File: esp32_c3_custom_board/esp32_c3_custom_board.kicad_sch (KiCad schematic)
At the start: 44 parts, among them IC1 ESP32-C3, IC2 GD25Q16CTEGR, J1 USB-C Connector, U1 ESD Protection, U2 SPX3819M5-L-3-3, Y1 830108208709_crystal

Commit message: .
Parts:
- IC1: footprint QFN50P500X500X90-33N-D -> ESP32-C3:QFN50P500X500X90-33N-D
- IC2: footprint SOIC127P600X175-8N -> GD25Q16CTEGR:SOIC127P600X175-8N
- J1: footprint GSB1C41110SSHR -> GSB1C41110SSHR:GSB1C41110SSHR
- S1: footprint 434781025816 -> 434781025816:434781025816
- U1: footprint Package_TO_SOT_SMD:SOT-666 -> USBLC6-2SC6:SOT95P280X145-6N
- U2: footprint Package_TO_SOT_SMD:SOT-23-5 -> SPX3819M5-L-3-3_TR:SOT95P280X145-5N
- Y1: footprint 830108208709 -> 830108208709:830108208709
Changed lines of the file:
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@@
       (effects (font (size 1.27 1.27)))
     )
-    (property "Footprint" "QFN50P500X500X90-33N-D" (at 240.03 154.61 0)
+    (property "Footprint" "ESP32-C3:QFN50P500X500X90-33N-D" (at 240.03 154.61 0)
       (effects (font (size 1.27 1.27)) (justify left top) hide)
     )
@@
       (effects (font (size 1 1)))
     )
-    (property "Footprint" "Package_TO_SOT_SMD:SOT-23-5" (at 115.57 28.575 0)
+    (property "Footprint" "SPX3819M5-L-3-3_TR:SOT95P280X145-5N" (at 115.57 28.575 0)
       (effects (font (size 1.27 1.27)) hide)
     )
@@
       (effects (font (size 1.27 1.27)) (justify left))
     )
-    (property "Footprint" "Package_TO_SOT_SMD:SOT-666" (at 97.79 172.72 0)
+    (property "Footprint" "USBLC6-2SC6:SOT95P280X145-6N" (at 97.79 172.72 0)
       (effects (font (size 1.27 1.27)) hide)
     )
@@
       (effects (font (size 1.27 1.27)))
     )
-    (property "Footprint" "830108208709" (at 246.38 233.35 0)
+    (property "Footprint" "830108208709:830108208709" (at 246.38 233.35 0)
       (effects (font (size 1.27 1.27)) (justify left top) hide)
     )
@@
       (effects (font (size 1.27 1.27)))
     )
-    (property "Footprint" "GSB1C41110SSHR" (at 68.58 223.19 0)
+    (property "Footprint" "GSB1C41110SSHR:GSB1C41110SSHR" (at 68.58 223.19 0)
       (effects (font (size 1.27 1.27)) (justify left top) hide)
     )
@@
       (effects (font (size 1.27 1.27)) (justify left))
     )
-    (property "Footprint" "434781025816" (at 196.85 187.63 0)
+    (property "Footprint" "434781025816:434781025816" (at 196.85 187.63 0)
       (effects (font (size 1.27 1.27)) (justify left top) hide)
     )
@@
       (effects (font (size 1.27 1.27)))
     )
-    (property "Footprint" "SOIC127P600X175-8N" (at 68.58 185.09 0)
-      (effects (font (size 1.27 1.27)) (justify left top) hide)
-    )
+    (property "Footprint" "GD25Q16CTEGR:SOIC127P600X175-8N" (at 68.58 185.09 0)
+      (effects (font (size 1.27 1.27)) (justify left top) hide)
+    )

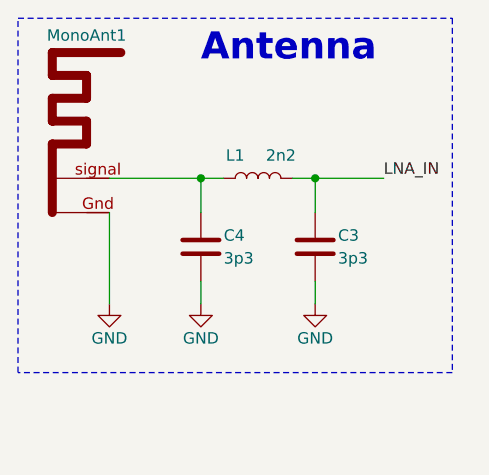
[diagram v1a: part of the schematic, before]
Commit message: .
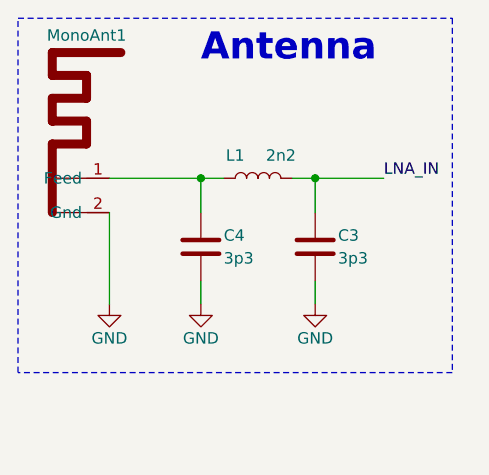
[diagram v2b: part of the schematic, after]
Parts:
- C1, C10, C11, C12, C13, C14, C15, C16, C2, C3, C4, C5, C6, C7, C8, C9: footprint (none) -> Capacitor_SMD:C_0201_0603Metric
- D1, D2: footprint (none) -> ASCKCF00-AP5R5010402:ASCKCF00AP5R5010402
- L1, L2: footprint (none) -> Inductor_SMD:L_0603_1608Metric
- MonoAnt1: footprint (none) -> Footprint_Lib:Mono_Ant
- R1, R10, R11, R12, R13, R14, R15, R2, R3, R4, R5, R6, R7, R8, R9: footprint (none) -> Resistor_SMD:R_0201_0603Metric
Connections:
- net GND: now also MonoAnt1.2 (Gnd); no longer MonoAnt1.Gnd
- net at C4.1, L1.1: now also MonoAnt1.1 (Feed); no longer MonoAnt1.signal
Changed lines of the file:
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@@
       (effects (font (size 1.27 1.27)) (justify left))
     )
-    (property "Footprint" "" (at 154.432 87.63 90)
+    (property "Footprint" "Resistor_SMD:R_0201_0603Metric" (at 154.432 87.63 90)
       (effects (font (size 1.27 1.27)) hide)
     )
@@
       (effects (font (size 1.27 1.27)) (justify left))
     )
-    (property "Footprint" "" (at 75.8952 45.72 0)
+    (property "Footprint" "Capacitor_SMD:C_0201_0603Metric" (at 75.8952 45.72 0)
       (effects (font (size 1.27 1.27)) hide)
     )
@@
       (effects (font (size 1.27 1.27)) (justify left))
     )
-    (property "Footprint" "" (at 100.0252 44.45 0)
+    (property "Footprint" "Capacitor_SMD:C_0201_0603Metric" (at 100.0252 44.45 0)
       (effects (font (size 1.27 1.27)) hide)
     )
@@
       (effects (font (size 1.27 1.27)) (justify left))
     )
-    (property "Footprint" "" (at 139.3952 46.99 0)
+    (property "Footprint" "Capacitor_SMD:C_0201_0603Metric" (at 139.3952 46.99 0)
       (effects (font (size 1.27 1.27)) hide)
     )
@@
       (effects (font (size 1.27 1.27)) (justify left))
     )
-    (property "Footprint" "" (at 101.2952 88.9 0)
+    (property "Footprint" "Capacitor_SMD:C_0201_0603Metric" (at 101.2952 88.9 0)
       (effects (font (size 1.27 1.27)) hide)
     )
@@
       (effects (font (size 1.27 1.27)))
     )
-    (property "Footprint" "" (at 250.19 76.708 90)
+    (property "Footprint" "Resistor_SMD:R_0201_0603Metric" (at 250.19 76.708 90)
       (effects (font (size 1.27 1.27)) hide)
     )
@@
       (effects (font (size 1.27 1.27)) (justify left))
     )
-    (property "Footprint" "" (at 36.5252 45.72 0)
+    (property "Footprint" "Capacitor_SMD:C_0201_0603Metric" (at 36.5252 45.72 0)
       (effects (font (size 1.27 1.27)) hide)
     )
@@
       (effects (font (size 1.27 1.27)) (justify left))
     )
-    (property "Footprint" "" (at 240.03 35.8648 0)
+    (property "Footprint" "Capacitor_SMD:C_0201_0603Metric" (at 240.03 35.8648 0)
       (effects (font (size 1.27 1.27)) hide)
     )
@@
       (effects (font (size 1.27 1.27)))
     )
-    (property "Footprint" "" (at 41.91 34.29 0)
+    (property "Footprint" "Inductor_SMD:L_0603_1608Metric" (at 41.91 34.29 0)
       (effects (font (size 1.27 1.27)) hide)
     )
@@
       (effects (font (size 1.27 1.27)) (justify right))
     )
-    (property "Footprint" "" (at 174.498 38.1 90)
+    (property "Footprint" "Resistor_SMD:R_0201_0603Metric" (at 174.498 38.1 90)
       (effects (font (size 1.27 1.27)) hide)
     )
@@
       (effects (font (size 1.27 1.27)) (justify left))
     )
-    (property "Footprint" "" (at 260.0452 92.71 0)
+    (property "Footprint" "Capacitor_SMD:C_0201_0603Metric" (at 260.0452 92.71 0)
       (effects (font (size 1.27 1.27)) hide)
     )
@@
       (effects (font (size 1.27 1.27)) (justify left))
     )
-    (property "Footprint" "" (at 75.8952 90.17 0)
+    (property "Footprint" "Capacitor_SMD:C_0201_0603Metric" (at 75.8952 90.17 0)
       (effects (font (size 1.27 1.27)) hide)
     )
@@
       (effects (font (size 1.27 1.27)) (justify left))
     )
-    (property "Footprint" "" (at 32.512 175.26 90)
+    (property "Footprint" "Resistor_SMD:R_0201_0603Metric" (at 32.512 175.26 90)
       (effects (font (size 1.27 1.27)) hide)
     )
@@
       (effects (font (size 1.27 1.27)) (justify left))
     )
-    (property "Footprint" "" (at 126.6952 46.99 0)
+    (property "Footprint" "Capacitor_SMD:C_0201_0603Metric" (at 126.6952 46.99 0)
       (effects (font (size 1.27 1.27)) hide)
     )
@@
       (effects (font (size 1.27 1.27)))
     )
-    (property "Footprint" "" (at 250.19 81.788 90)
+    (property "Footprint" "Resistor_SMD:R_0201_0603Metric" (at 250.19 81.788 90)
       (effects (font (size 1.27 1.27)) hide)
     )
@@
       (effects (font (size 1.27 1.27)))
     )
-    (property "Footprint" "" (at 151.13 34.29 0)
+    (property "Footprint" "ASCKCF00-AP5R5010402:ASCKCF00AP5R5010402" (at 151.13 34.29 0)
       (effects (font (size 1.27 1.27)) hide)
     )
@@
       (effects (font (size 1.27 1.27)))
     )
-    (property "Footprint" "" (at 194.31 147.828 90)
+    (property "Footprint" "Resistor_SMD:R_0201_0603Metric" (at 194.31 147.828 90)
       (effects (font (size 1.27 1.27)) hide)
     )
@@
       (effects (font (size 1.27 1.27)) (justify left))
     )
-    (property "Footprint" "" (at 174.9552 93.98 0)
+    (property "Footprint" "Capacitor_SMD:C_0201_0603Metric" (at 174.9552 93.98 0)
       (effects (font (size 1.27 1.27)) hide)
     )
@@
       (effects (font (size 1.27 1.27)) (justify left))
     )
-    (property "Footprint" "" (at 245.11 40.9448 0)
+    (property "Footprint" "Capacitor_SMD:C_0201_0603Metric" (at 245.11 40.9448 0)
       (effects (font (size 1.27 1.27)) hide)
     )
@@
       (effects (font (size 1.27 1.27)) (justify left))
     )
-    (property "Footprint" "" (at 172.212 80.01 90)
+    (property "Footprint" "Resistor_SMD:R_0201_0603Metric" (at 172.212 80.01 90)
       (effects (font (size 1.27 1.27)) hide)
     )
@@
       (effects (font (size 1.27 1.27)) (justify left))
     )
-    (property "Footprint" "" (at 106.3752 99.06 0)
+    (property "Footprint" "Capacitor_SMD:C_0201_0603Metric" (at 106.3752 99.06 0)
       (effects (font (size 1.27 1.27)) hide)
     )
@@
       (effects (font (size 1.27 1.27)))
     )
-    (property "Footprint" "" (at 250.19 71.628 90)
+    (property "Footprint" "Resistor_SMD:R_0201_0603Metric" (at 250.19 71.628 90)
       (effects (font (size 1.27 1.27)) hide)
     )
@@
       (effects (font (size 1.27 1.27)))
     )
-    (property "Footprint" "" (at 172.72 29.21 0)
+    (property "Footprint" "ASCKCF00-AP5R5010402:ASCKCF00AP5R5010402" (at 172.72 29.21 0)
       (effects (font (size 1.27 1.27)) hide)
     )
@@
       (effects (font (size 1.27 1.27)))
     )
-    (property "Footprint" "" (at 250.19 84.328 90)
+    (property "Footprint" "Resistor_SMD:R_0201_0603Metric" (at 250.19 84.328 90)
       (effects (font (size 1.27 1.27)) hide)
     )
@@
       (effects (font (size 1.27 1.27)) (justify left))
     )
-    (property "Footprint" "" (at 88.5952 45.72 0)
+    (property "Footprint" "Capacitor_SMD:C_0201_0603Metric" (at 88.5952 45.72 0)
       (effects (font (size 1.27 1.27)) hide)
     )
@@
       (effects (font (size 1.27 1.27)) (justify left))
     )
-    (property "Footprint" "" (at 205.4352 146.05 0)
+    (property "Footprint" "Capacitor_SMD:C_0201_0603Metric" (at 205.4352 146.05 0)
       (effects (font (size 1.27 1.27)) hide)
     )
@@
       (effects (font (size 1.27 1.27)) (justify right))
     )
-    (property "Footprint" "" (at 159.258 41.91 90)
+    (property "Footprint" "Resistor_SMD:R_0201_0603Metric" (at 159.258 41.91 90)
       (effects (font (size 1.27 1.27)) hide)
     )
@@
       (effects (font (size 1.27 1.27)) (justify left))
     )
-    (property "Footprint" "" (at 49.2252 45.72 0)
+    (property "Footprint" "Capacitor_SMD:C_0201_0603Metric" (at 49.2252 45.72 0)
       (effects (font (size 1.27 1.27)) hide)
     )
@@
       (effects (font (size 1.27 1.27)) (justify left))
     )
-    (property "Footprint" "" (at 144.272 86.36 90)
+    (property "Footprint" "Resistor_SMD:R_0201_0603Metric" (at 144.272 86.36 90)
       (effects (font (size 1.27 1.27)) hide)
     )
@@
       (effects (font (size 1.27 1.27)) (justify left))
     )
-    (property "Footprint" "" (at 47.498 175.26 90)
+    (property "Footprint" "Resistor_SMD:R_0201_0603Metric" (at 47.498 175.26 90)
       (effects (font (size 1.27 1.27)) hide)
     )
@@
       (effects (font (size 1.27 1.27)))
     )
-    (property "Footprint" "" (at 81.28 34.29 0)
+    (property "Footprint" "Inductor_SMD:L_0603_1608Metric" (at 81.28 34.29 0)
       (effects (font (size 1.27 1.27)) hide)
     )
@@
       (effects (font (size 1.27 1.27)))
     )
-    (property "Footprint" "" (at 24.13 31.75 0)
+    (property "Footprint" "Footprint_Lib:Mono_Ant" (at 24.13 31.75 0)
       (effects (font (size 1.27 1.27)) hide)
     )
@@
       (effects (font (size 1.27 1.27)) hide)
     )
-    (pin "signal")
-    (pin "Gnd")
+    (pin "2")
+    (pin "1")
     (instances
       (project "esp32_c3_custom_board"
@@
       (effects (font (size 1.27 1.27)))
     )
-    (property "Footprint" "" (at 250.19 74.168 90)
+    (property "Footprint" "Resistor_SMD:R_0201_0603Metric" (at 250.19 74.168 90)
       (effects (font (size 1.27 1.27)) hide)
     )
@@
       (effects (font (size 1.27 1.27)) (justify left))
     )
-    (property "Footprint" "" (at 265.1252 146.05 0)
+    (property "Footprint" "Capacitor_SMD:C_0201_0603Metric" (at 265.1252 146.05 0)
       (effects (font (size 1.27 1.27)) hide)
     )
@@
       (effects (font (size 1.27 1.27)))
     )
-    (property "Footprint" "" (at 230.378 48.26 90)
+    (property "Footprint" "Resistor_SMD:R_0201_0603Metric" (at 230.378 48.26 90)
       (effects (font (size 1.27 1.27)) hide)
     )
@@
       (effects (font (size 1.27 1.27)))
     )
-    (property "Footprint" "" (at 232.918 48.26 90)
-      (effects (font (size 1.27 1.27)) hide)
-    )
+    (property "Footprint" "Resistor_SMD:R_0201_0603Metric" (at 232.918 48.26 90)
+      (effects (font (size 1.27 1.27)) hide)
+    )

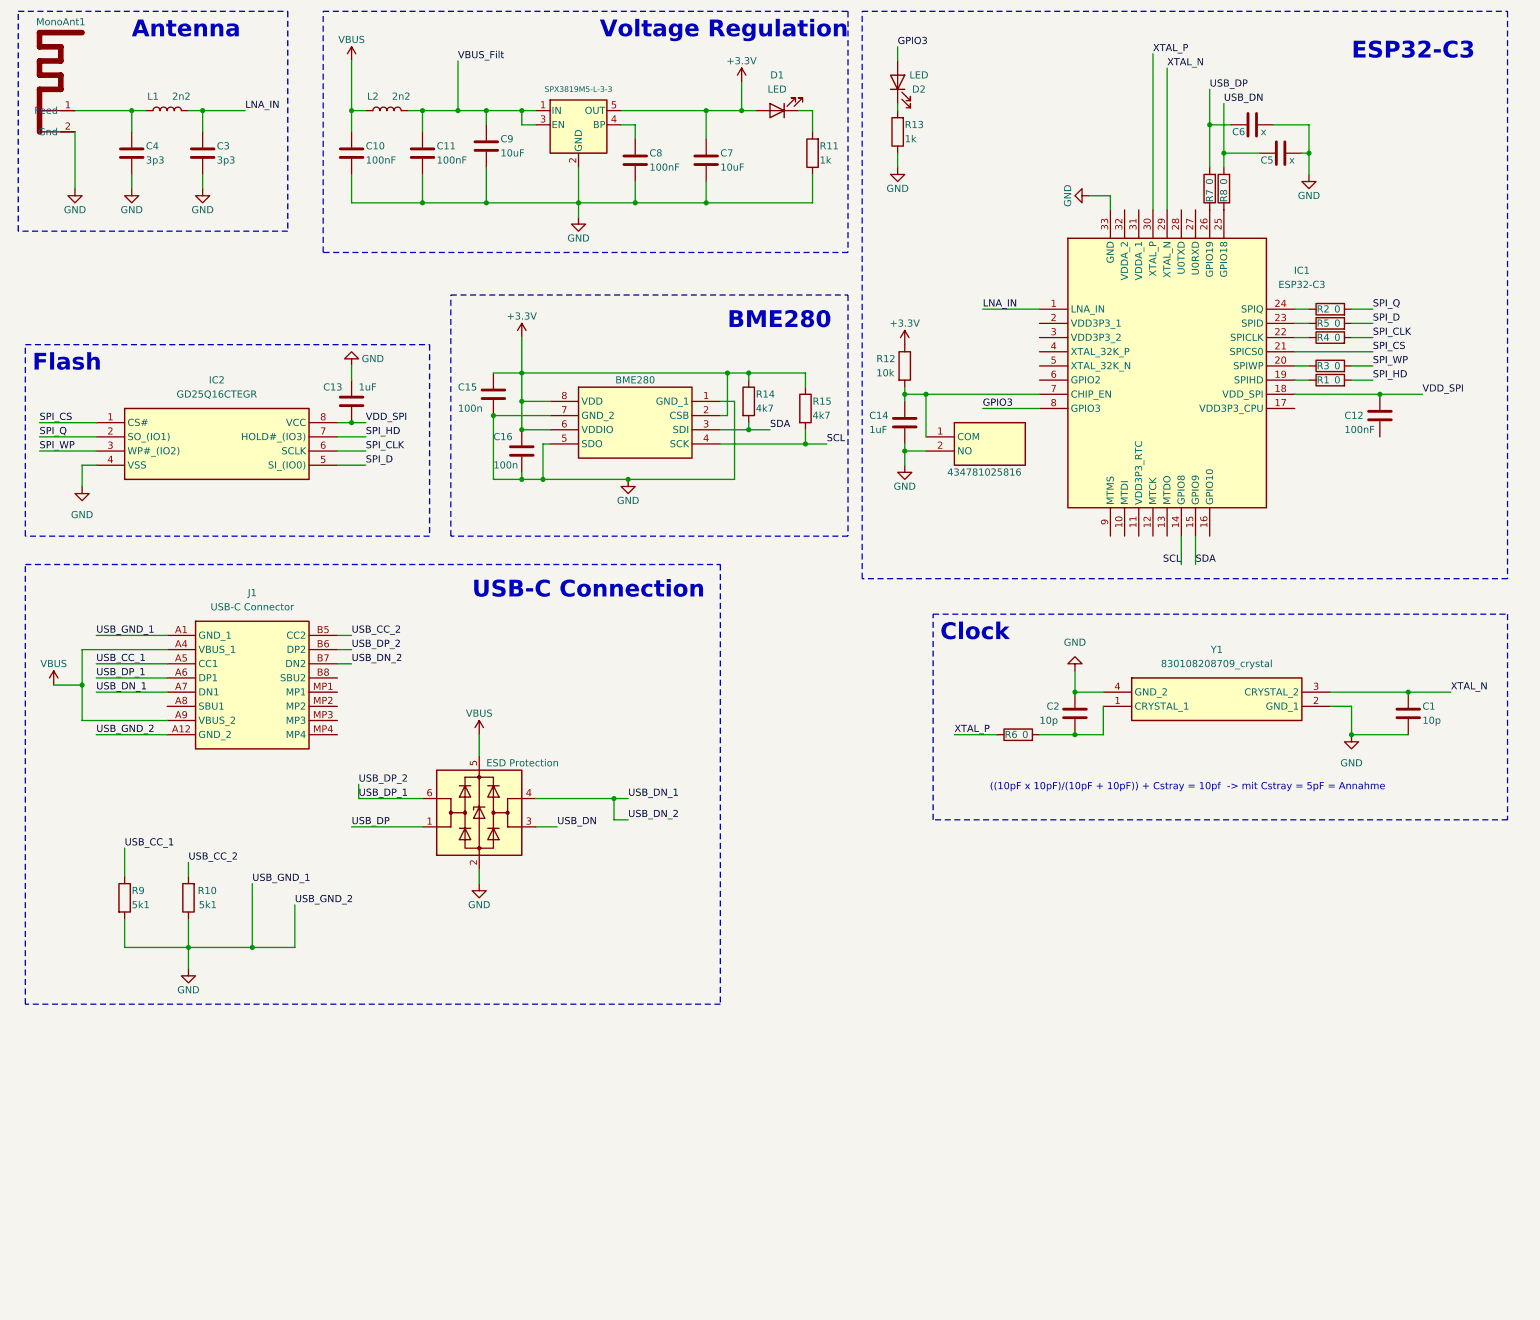
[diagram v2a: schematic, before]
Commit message: .
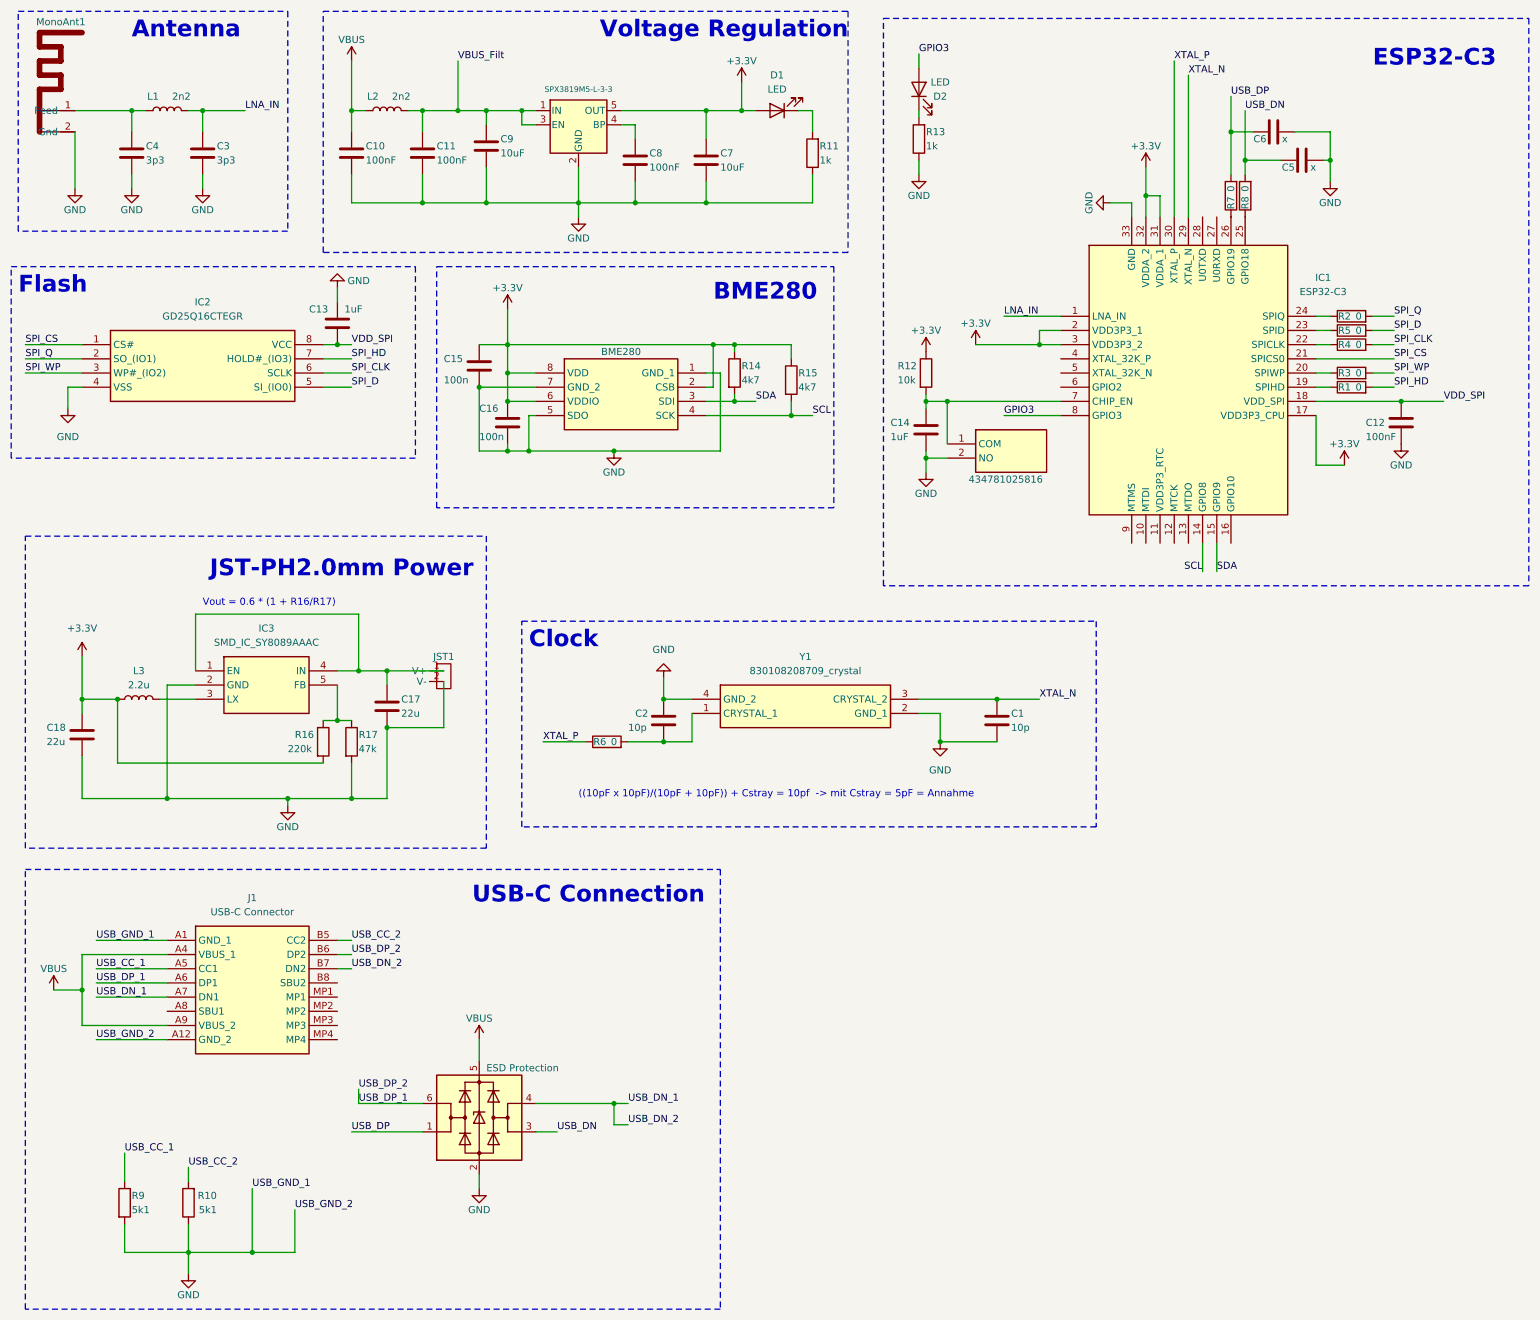
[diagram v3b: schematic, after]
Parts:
- added C17, C18: 22u, Capacitor_SMD:C_0201_0603Metric, symbol Device:C
- added IC3: SMD_IC_SY8089AAAC, SY8089AAAC:SOT95P285X140-5N, symbol SMD_IC_SY8089AAAC:SMD_IC_SY8089AAAC
- added JST1: ~, JST_Connectors:JST-PH2.0mm, symbol JST_Connectors:JST-PH2.0mm
- added L3: 2.2u, Inductor_SMD:L_0201_0603Metric, symbol Device:L
- added R16: 220k, Resistor_SMD:R_0201_0603Metric, symbol Device:R
- added R17: 47k, Resistor_SMD:R_0201_0603Metric, symbol Device:R
- L1, L2: footprint Inductor_SMD:L_0603_1608Metric -> Inductor_SMD:L_0201_0603Metric
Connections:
- net +3.3V: now also IC1.17 (VDD3P3_CPU), IC1.2 (VDD3P3_1), IC1.3 (VDD3P3_2), IC1.31 (VDDA_1), IC1.32 (VDDA_2), C18.1, L3.1, R16.2
- net GND: now also C12.2, C17.2, C18.2, IC3.2 (GND), JST1.2 (V-), R17.2
- new net: IC3.5 (FB), R16.1, R17.1
- new net: C17.1, IC3.1 (EN), IC3.4 (IN), JST1.1 (V+)
- new net: IC3.3 (LX), L3.2
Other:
- note added: "JST-PH2.0mm Power"
- note added: "Vout = 0.6 * (1 + R16/R17)"
- moved on the sheet: C1, C12, C13, C14, C15, C16, C2, C5, C6, D2, IC1, IC2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
